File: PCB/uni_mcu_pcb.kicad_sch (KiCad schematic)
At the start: 5 parts

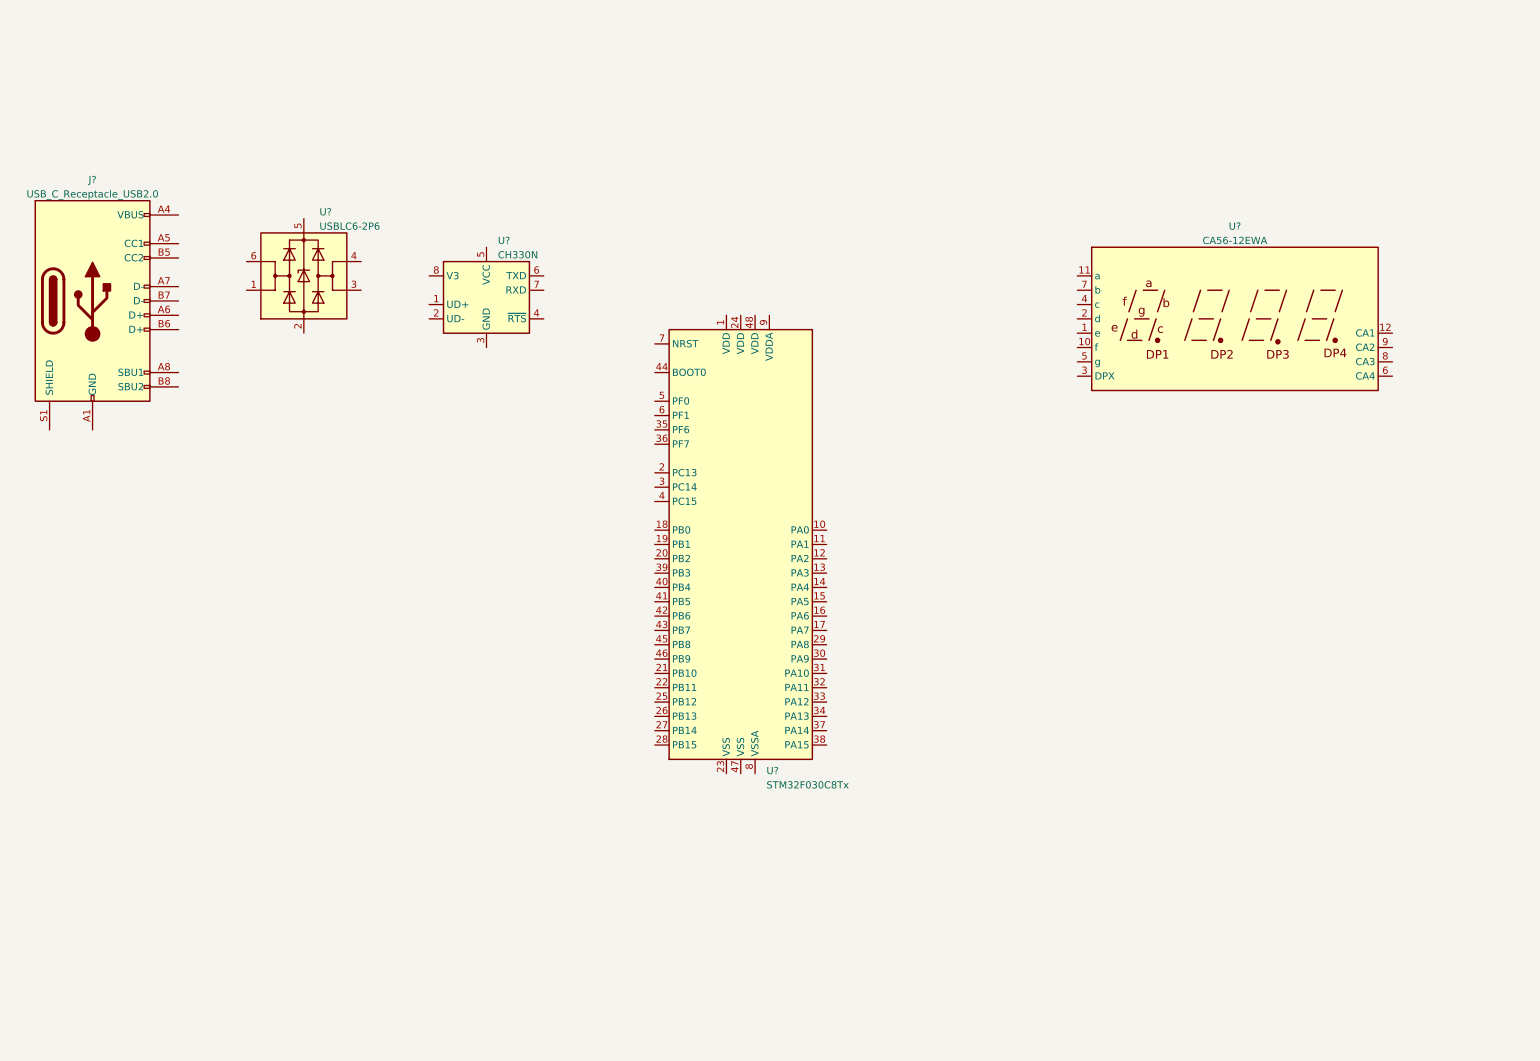
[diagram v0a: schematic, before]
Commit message: Схемотехника разработана на 80%
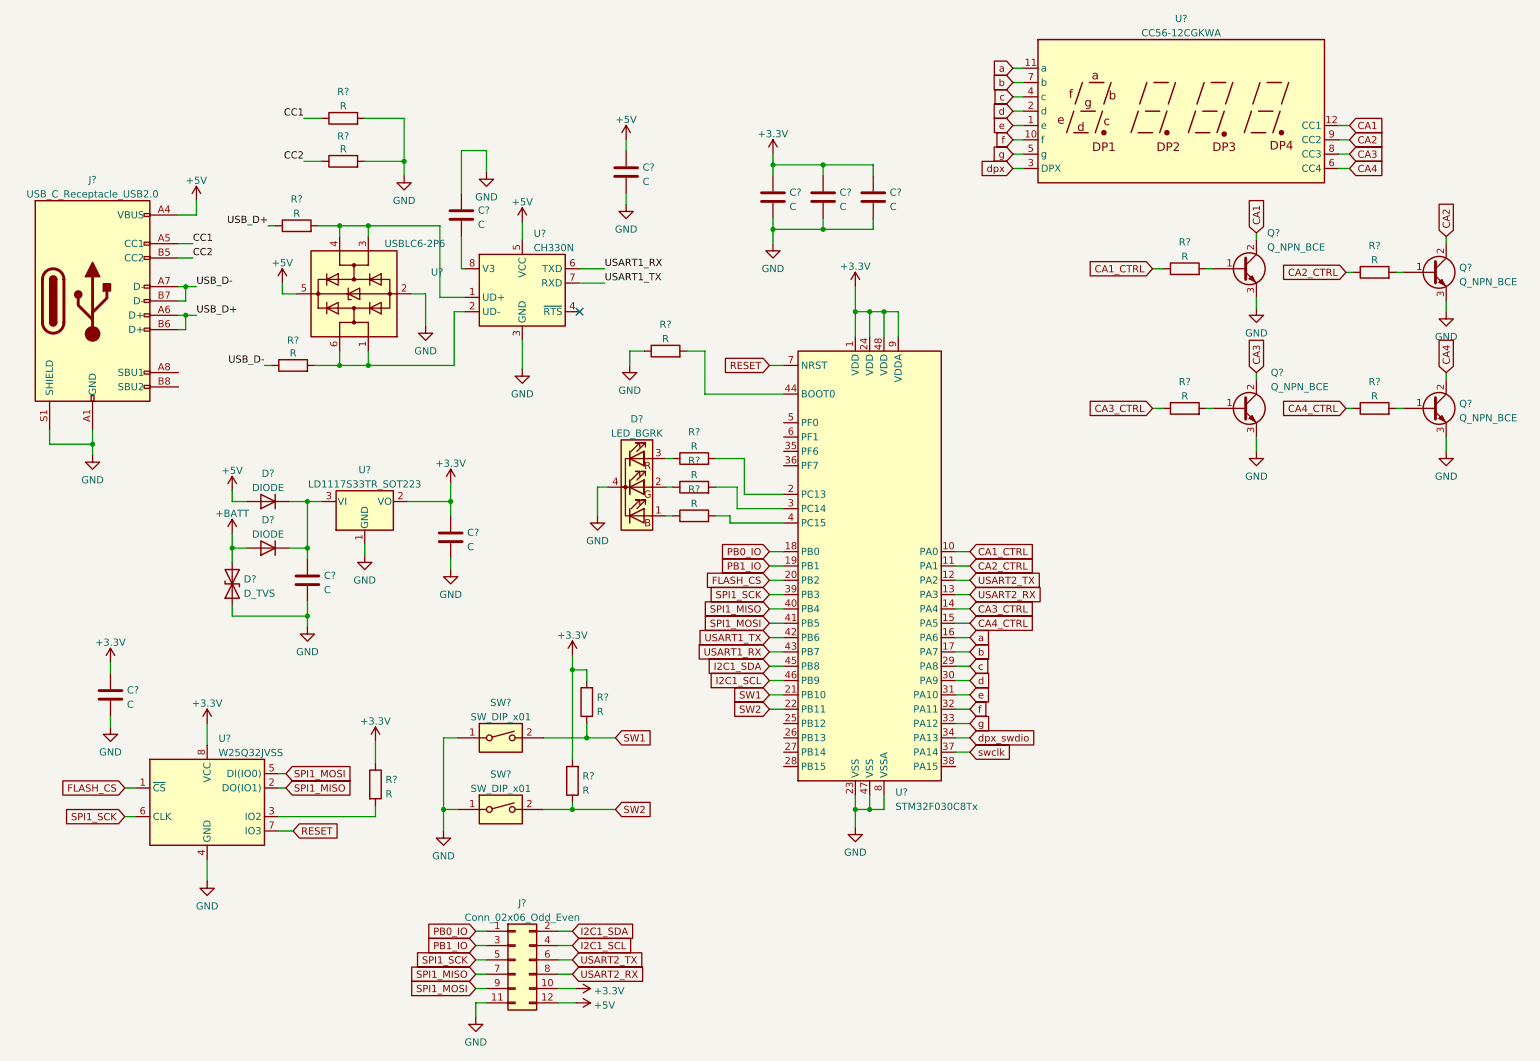
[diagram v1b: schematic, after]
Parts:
- removed U?: CA56-12EWA, Display_7Segment:CA56-12EWA, symbol Display_Character:CA56-12EWA
- added C? (x8): C, symbol Device:C
- added D?: LED_BGRK, symbol Device:LED_BGRK
- added D?: D_TVS, symbol Device:D_TVS
- added D? (x2): DIODE, symbol Simulation_SPICE:DIODE
- added J?: Conn_02x06_Odd_Even, symbol Connector_Generic:Conn_02x06_Odd_Even
- added Q? (x4): Q_NPN_BCE, symbol Device:Q_NPN_BCE
- added R? (x15): R, symbol Device:R
- added SW? (x2): SW_DIP_x01, symbol Switch:SW_DIP_x01
- added U?: LD1117S33TR_SOT223, Package_TO_SOT_SMD:SOT-223-3_TabPin2, symbol Regulator_Linear:LD1117S33TR_SOT223
- added U?: W25Q32JVSS, Package_SO:SOIC-8_5.23x5.23mm_P1.27mm, symbol Memory_Flash:W25Q32JVSS
- added U?: CC56-12CGKWA, Display_7Segment:CA56-12CGKWA, symbol Display_Character:CC56-12CGKWA
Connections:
- net GND: now reaches J?.A1 (GND), J?.A12 (GND), J?.B1 (GND), J?.B12 (GND)
- net GND: now also J?.S1 (SHIELD), U?.2 (GND), U?.23 (VSS), U?.3 (GND), U?.47 (VSS), U?.8 (VSSA), C?.1, C?.2, C?.2, C?.2, C?.2, C?.2, C?.2, C?.2, D?.1 (A1), D?.4 (K), J?.11 (Pin_11), Q?.3 (E), Q?.3 (E), Q?.3 (E), Q?.3 (E), R?.1, R?.2, R?.2, SW?.1, SW?.1, U?.1 (GND), U?.4 (GND)
- net +5V: now reaches J?.A4 (VBUS), J?.A9 (VBUS), J?.B4 (VBUS), J?.B9 (VBUS)
- net +5V: now also U?.5 (VBUS), U?.5 (VCC), C?.1, D?.1 (A), J?.12 (Pin_12)
- net CC1: now reaches J?.A5 (CC1)
- net CC1: now also R?.1
- net USB_D+: now reaches J?.A6 (D+)
- net USB_D+: now also J?.B6 (D+), R?.1
- net USB_D-: now reaches J?.A7 (D-)
- net USB_D-: now also J?.B7 (D-), R?.1
- net CC2: now reaches J?.B5 (CC2)
- net CC2: now also R?.1
- net at U?.1 (I/O1): now also U?.2 (UD-), U?.6 (I/O1), R?.2
- net at U?.3 (I/O2): now also U?.1 (UD+), U?.4 (I/O2), R?.2
- net USART1_RX: now reaches U?.6 (TXD)
- net USART1_RX: now also U?.43 (PB7)
- net USART1_TX: now reaches U?.7 (RXD)
- net USART1_TX: now also U?.42 (PB6)
- net at U?.8 (V3): now also C?.2
- net +3V3: now reaches U?.1 (VDD)
- net +3V3: now also U?.24 (VDD), U?.48 (VDD), U?.9 (VDDA), C?.1, C?.1, C?.1, C?.1, C?.1, J?.10 (Pin_10), R?.1, R?.2, R?.2, U?.2 (VO), U?.8 (VCC)
- net CA1_CTRL: now reaches U?.10 (PA0)
- net CA1_CTRL: now also R?.1
- net CA2_CTRL: now reaches U?.11 (PA1)
- net CA2_CTRL: now also R?.1
- net USART2_TX: now reaches U?.12 (PA2)
- net USART2_TX: now also J?.6 (Pin_6)
- net USART2_RX: now reaches U?.13 (PA3)
- net USART2_RX: now also J?.8 (Pin_8)
- net CA3_CTRL: now reaches U?.14 (PA4)
- net CA3_CTRL: now also R?.1
- net CA4_CTRL: now reaches U?.15 (PA5)
- net CA4_CTRL: now also R?.1
- net a: now reaches U?.16 (PA6)
- net a: now also U?.11 (a)
- net b: now reaches U?.17 (PA7)
- net b: now also U?.7 (b)
- net PB0_IO: now reaches U?.18 (PB0)
- net PB0_IO: now also J?.1 (Pin_1)
- net PB1_IO: now reaches U?.19 (PB1)
- net PB1_IO: now also J?.3 (Pin_3)
- net at U?.2 (PC13): now also R?.2
- net FLASH_CS: now reaches U?.20 (PB2)
- net FLASH_CS: now also U?.1 (~{CS})
- net SW1: now reaches U?.21 (PB10)
- net SW1: now also R?.1, SW?.2
- net SW2: now reaches U?.22 (PB11)
- net SW2: now also R?.1, SW?.2
- net c: now reaches U?.29 (PA8)
- net c: now also U?.4 (c)
- net at U?.3 (PC14): now also R?.2
- net d: now reaches U?.30 (PA9)
- net d: now also U?.2 (d)
- net e: now reaches U?.31 (PA10)
- net e: now also U?.1 (e)
- net f: now reaches U?.32 (PA11)
- net f: now also U?.10 (f)
- net g: now reaches U?.33 (PA12)
- net g: now also U?.5 (g)
- net dpx_swdio: now reaches U?.34 (PA13)
- net swclk: now reaches U?.37 (PA14)
- net SPI1_SCK: now reaches U?.39 (PB3)
- net SPI1_SCK: now also J?.5 (Pin_5), U?.6 (CLK)
- net at U?.4 (PC15): now also R?.2
- net SPI1_MISO: now reaches U?.40 (PB4)
- net SPI1_MISO: now also J?.7 (Pin_7), U?.2 (DO(IO1))
- net SPI1_MOSI: now reaches U?.41 (PB5)
- net SPI1_MOSI: now also J?.9 (Pin_9), U?.5 (DI(IO0))
- net at U?.44 (BOOT0): now also R?.2
- net I2C1_SDA: now reaches U?.45 (PB8)
- net I2C1_SDA: now also J?.2 (Pin_2)
- net I2C1_SCL: now reaches U?.46 (PB9)
- net I2C1_SCL: now also J?.4 (Pin_4)
- net RESET: now reaches U?.7 (NRST)
- net RESET: now also U?.7 (IO3)
- new net: D?.3 (RA), R?.1
- new net: C?.1, D?.2 (K), D?.2 (K), U?.3 (VI)
- new net: D?.2 (GA), R?.1
- new net: Q?.1 (B), R?.2 (x4)
- new net: D?.1 (BA), R?.1
- new net: R?.2, U?.3 (IO2)
- new net +BATT: D?.1 (A), D?.2 (A2)
- new net CA1: Q?.2 (C), U?.12 (CC1)
- new net CA2: Q?.2 (C), U?.9 (CC2)
- new net CA3: Q?.2 (C), U?.8 (CC3)
- new net CA4: Q?.2 (C), U?.6 (CC4)
- new net dpx: U?.3 (DPX)
- no-connect marks 0 -> 1
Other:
- moved on the sheet: U?
